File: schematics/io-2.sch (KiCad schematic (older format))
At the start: 14 parts, among them J13 FDC Connector, J9 IDE Connector, U11 WD1772, U13 74LS574, U14 74LS574, U15 74LS245, U16 74LS245

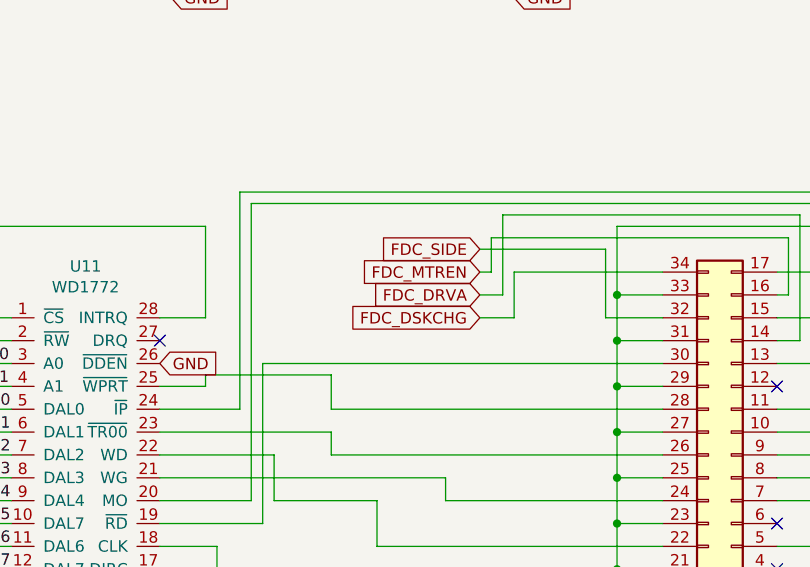
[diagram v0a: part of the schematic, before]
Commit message: additional fixups
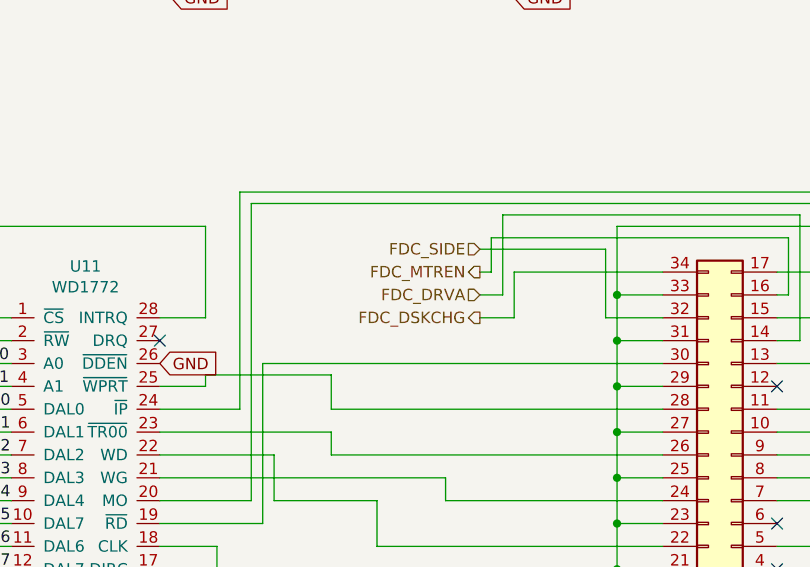
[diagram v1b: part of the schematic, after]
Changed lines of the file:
@@
 $Descr A4 11693 8268
 encoding utf-8
-Sheet 4 7
+Sheet 3 7
 Title ""
 Date ""
@@
 Wire Wire Line
 	4950 5250 4300 5250
-Text GLabel 4150 5450 0    50   Input ~ 0
-FDC_DSKCHG
 Wire Wire Line
 	4150 5350 4250 5350
@@
 Wire Wire Line
 	5550 5550 5550 5000
-Text GLabel 4150 5350 0    50   Input ~ 0
-FDC_DRVA
 Wire Wire Line
 	4200 5100 4200 5250
@@
 Wire Wire Line
 	5450 5350 5500 5350
-Text GLabel 4150 5250 0    50   Input ~ 0
-FDC_MTREN
 Wire Wire Line
 	4700 5150 4150 5150
@@
 Wire Wire Line
 	4950 5450 4700 5450
-Text GLabel 4150 5150 0    50   Input ~ 0
-FDC_SIDE
 Wire Wire Line
 	2600 6950 2950 6950
@@
 Text HLabel 1550 5050 0    50   Output ~ 0
 IRQ_HIGH
-Wire Wire Line
-	8350 2850 8850 2850
-Wire Wire Line
-	8350 2650 8850 2650
-Wire Wire Line
-	8350 2450 8850 2450
-Wire Wire Line
-	8350 2250 8850 2250
-Wire Wire Line
-	8350 2050 8850 2050
-Wire Wire Line
-	8350 1850 8850 1850
-Wire Wire Line
-	8350 1650 8850 1650
-Wire Bus Line
-	9650 2450 9650 2800
-Wire Bus Line
-	1850 5700 1850 5900
-Wire Bus Line
-	1850 5950 1850 6650
-Wire Bus Line
-	2300 950  2300 1950
-Wire Bus Line
-	1800 2650 1800 3950
-Wire Bus Line
-	8250 1450 8250 3100
-Wire Bus Line
-	8400 1350 8400 3000
-Wire Bus Line
-	3950 1050 3950 2450
-Wire Bus Line
-	3550 2450 3550 3550
-Wire Bus Line
-	5700 1050 5700 1950
-Wire Bus Line
-	5300 2650 5300 3950
 Text Notes 550  5000 0    50   ~ 0
 This is active high! >>>
@@
 Text HLabel 9500 3050 2    50   Input ~ 0
 IDE_CS1
+Text HLabel 4150 5150 0    50   Input ~ 0
+FDC_SIDE
+Text HLabel 4150 5250 0    50   Output ~ 0
+FDC_MTREN
+Text HLabel 4150 5350 0    50   Input ~ 0
+FDC_DRVA
+Text HLabel 4150 5450 0    50   Output ~ 0
+FDC_DSKCHG
+Wire Wire Line
+	8350 2850 8850 2850
+Wire Wire Line
+	8350 2650 8850 2650
+Wire Wire Line
+	8350 2450 8850 2450
+Wire Wire Line
+	8350 2250 8850 2250
+Wire Wire Line
+	8350 2050 8850 2050
+Wire Wire Line
+	8350 1850 8850 1850
+Wire Wire Line
+	8350 1650 8850 1650
+Wire Bus Line
+	9650 2450 9650 2800
+Wire Bus Line
+	1850 5700 1850 5900
+Wire Bus Line
+	1850 5950 1850 6650
+Wire Bus Line
+	2300 950  2300 1950
+Wire Bus Line
+	1800 2650 1800 3950
+Wire Bus Line
+	8250 1450 8250 3100
+Wire Bus Line
+	8400 1350 8400 3000
+Wire Bus Line
+	3950 1050 3950 2450
+Wire Bus Line
+	3550 2450 3550 3550
+Wire Bus Line
+	5700 1050 5700 1950
+Wire Bus Line
+	5300 2650 5300 3950
 $EndSCHEMATC
